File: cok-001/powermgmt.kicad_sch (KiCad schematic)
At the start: 87 parts, among them J6004 +12V_MAIN, J6005 +5V_EVER, Q6001 FDQ7238AS, Q6002 FDQ7238AS, Q6003 DTC144E, Q6004 SI3493, Q6006 UMH2NTN, Q6007 SI3493, Q6008 SI3493, Q6009 UMH2NTN, Q6010 SI4943, Q6012 Si3460DV, U6003 MB39A, U6004 PST3642UL, U6005 NCP511SN33T1G, U6006 NCP511SN18T1, U6007 TPS73101DBV, U6008 NCP511SN18T1, U6009 NCP511SN33T1G, U6011 NCP511, U6012 MM3141, U6013 MM1562, U6014 MM1591, U6017 BD3521, U6019 NCP511SN18T1, U6021 MM1591, U6022 MM1593, U6023 PST3642UL

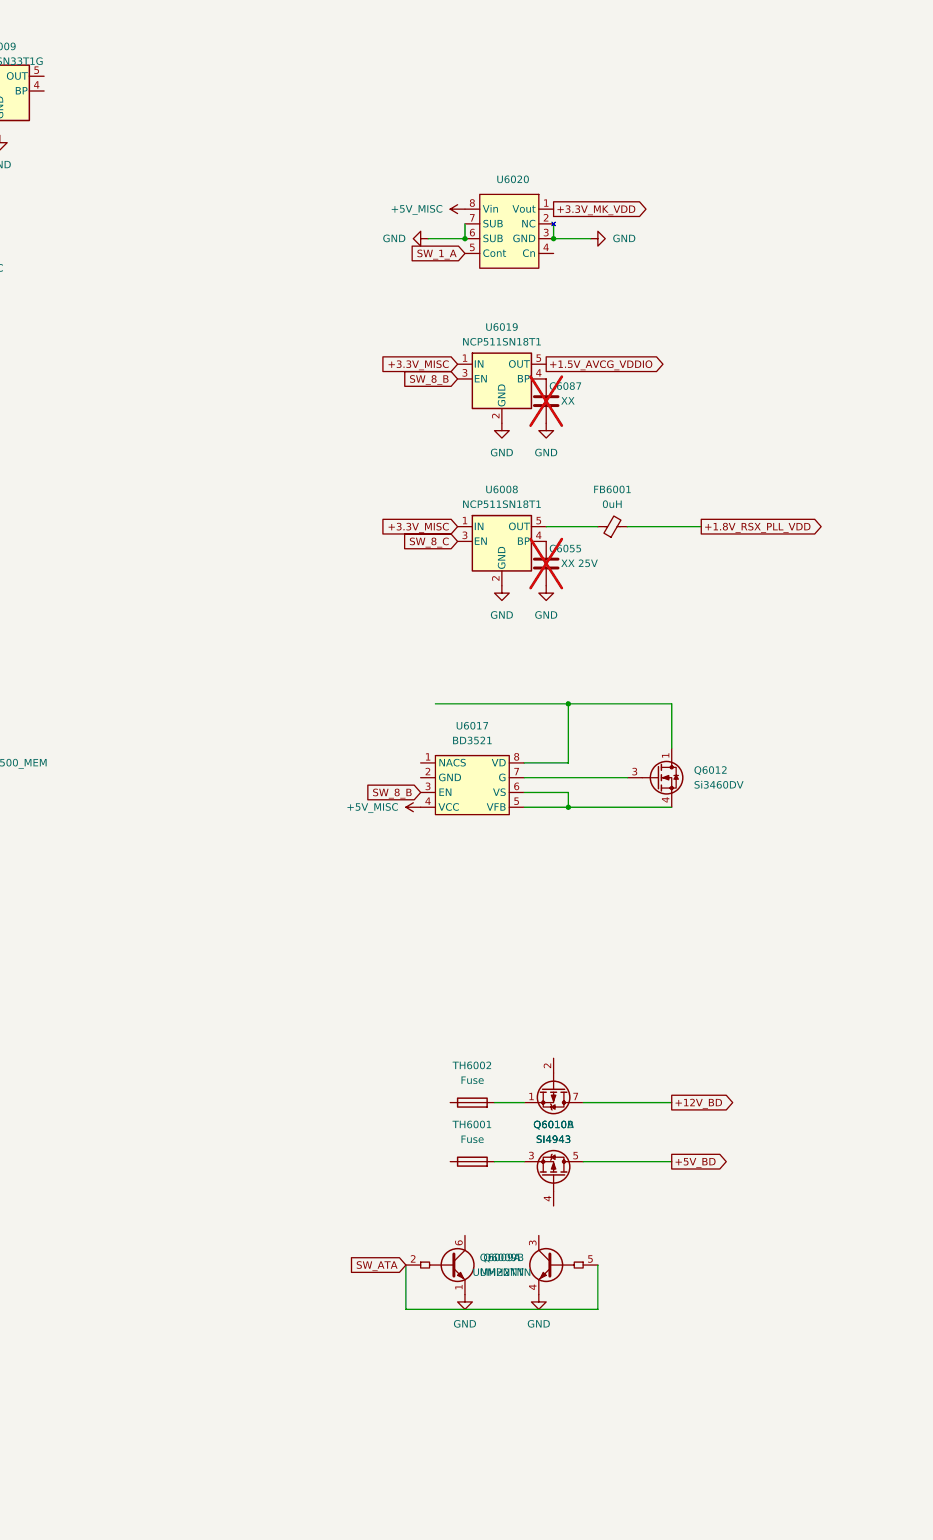
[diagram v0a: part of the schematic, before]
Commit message: caps
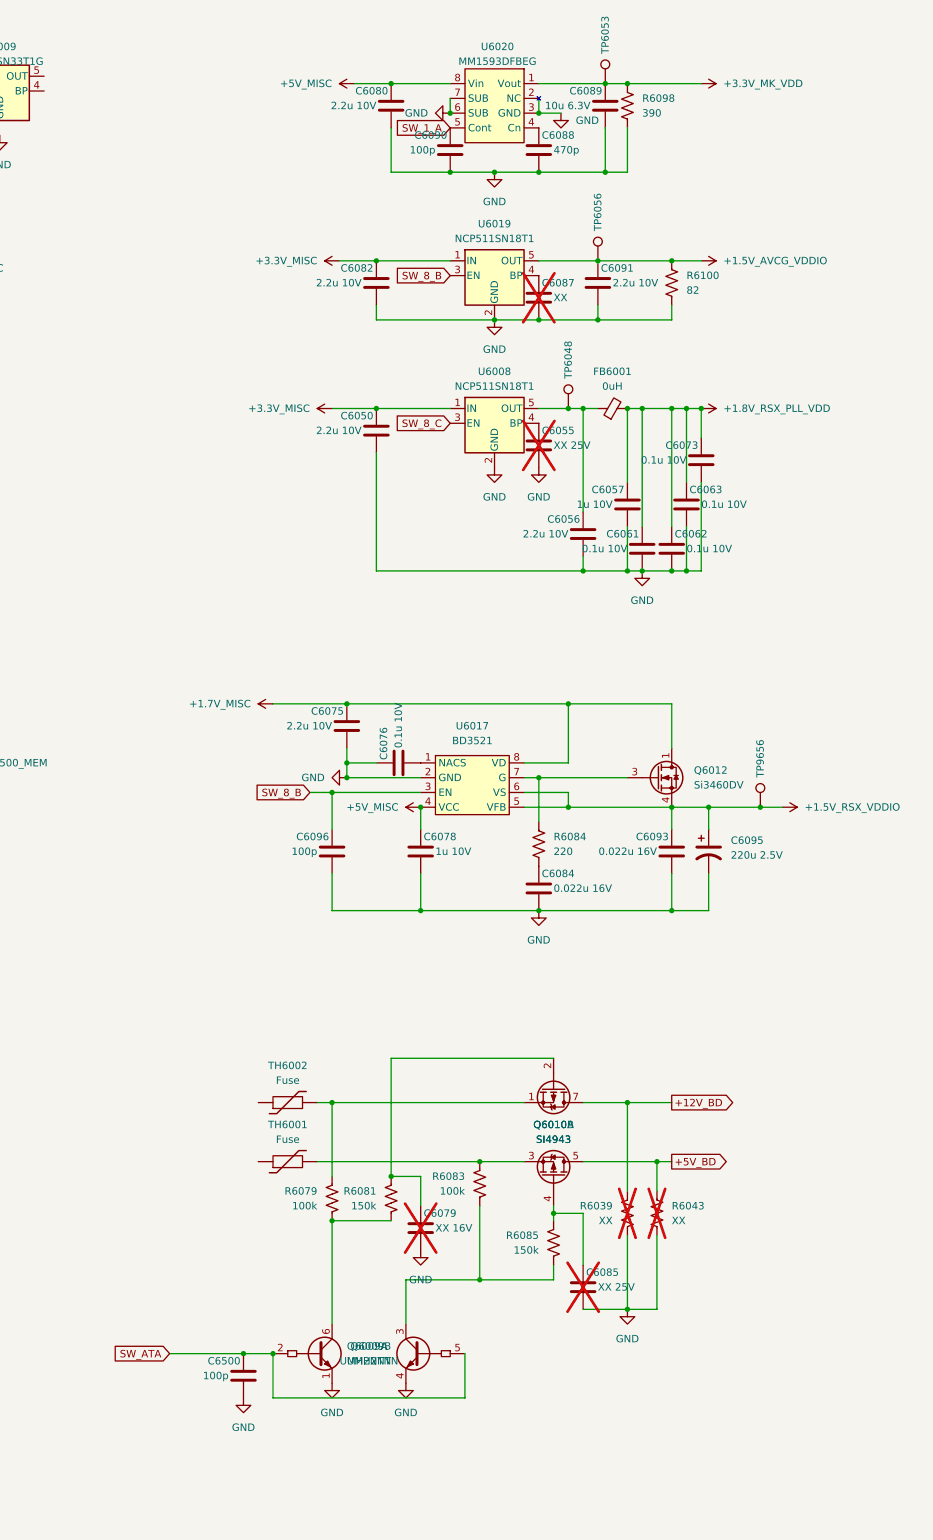
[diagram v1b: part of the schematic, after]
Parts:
- added C6050, C6056, C6075, C6080, C6082, C6091: 2.2u 10V, Capacitor_SMD:C_0805_2012Metric, symbol Device:C
- added C6057, C6078: 1u 10V, Capacitor_SMD:C_0402_1005Metric, symbol Device:C
- added C6061, C6062, C6063, C6073, C6076: 0.1u 10V, Capacitor_SMD:C_0402_1005Metric, symbol Device:C
- added C6079: XX 16V, Capacitor_SMD:C_0402_1005Metric, symbol Device:C
- added C6084, C6093: 0.022u 16V, Capacitor_SMD:C_0402_1005Metric, symbol Device:C
- added C6085: XX 25V, Capacitor_SMD:C_0402_1005Metric, symbol Device:C
- added C6088: 470p, Capacitor_SMD:C_0402_1005Metric, symbol Device:C
- added C6089: 10u 6.3V, Capacitor_SMD:C_0805_2012Metric, symbol Device:C
- added C6090, C6096, C6500: 100p, Capacitor_SMD:C_0402_1005Metric, symbol Device:C
- added C6095: 220u 2.5V, Capacitor_Tantalum_SMD:CP_EIA-3528-21_Kemet-B, symbol Device:C_Polarized_US
- added R6039, R6043: XX, Resistor_SMD:R_0402_1005Metric, symbol Device:R_US
- added R6079, R6083: 100k, Resistor_SMD:R_0402_1005Metric, symbol Device:R_US
- added R6081, R6085: 150k, Resistor_SMD:R_0402_1005Metric, symbol Device:R_US
- added R6084: 220, Resistor_SMD:R_0402_1005Metric, symbol Device:R_US
- added R6098: 390, Resistor_SMD:R_0402_1005Metric, symbol Device:R_US
- added R6100: 82, Resistor_SMD:R_0402_1005Metric, symbol Device:R_US
- added TP6048, TP6053, TP6056, TP9656: TestPoint, TestPoint:TestPoint_Pad_1.0x1.0mm, symbol Connector:TestPoint
- TH6001, TH6002: symbol Device:Fuse -> Device:Thermistor
- U6020: value ~ -> MM1593DFBEG
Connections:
- net +1.5V_AVCG_VDDIO: now also C6091.1, R6100.2, TP6056.1
- net +1.8V_RSX_PLL_VDD: now also C6057.1, C6061.1, C6062.1, C6063.1, C6073.1
- net +12V_BD: now also R6039.2
- net +3.3V_MISC: now also C6050.1, C6082.1
- net +3.3V_MK_VDD: now also C6089.1, R6098.2, TP6053.1
- net +5V_BD: now also R6043.2
- net +5V_MISC: now also C6078.1, C6080.1
- net GND: now also U6017.2 (GND), C6050.2, C6056.2, C6057.2, C6061.2, C6062.2, C6063.2, C6073.2, C6075.2, C6076.1, C6078.2, C6079.2, C6080.2, C6082.2, C6084.2, C6085.2, C6088.2, C6089.2, C6090.2, C6091.2, C6093.2, C6095.2, C6096.2, C6500.2, R6039.1, R6043.1, R6098.1, R6100.1
- net SW_1_A: now also C6090.1
- net SW_8_B: now also C6096.1
- net SW_ATA: now also C6500.1
- net +1.7V_MISC: now reaches Q6012.1 (D), Q6012.2 (D), Q6012.5 (D), Q6012.6 (D), U6017.8 (VD)
- net +1.7V_MISC: now also C6075.1
- net at Q6012.3 (G), U6017.7 (G): now also R6084.2
- net +1.5V_RSX_VDDIO: now reaches Q6012.4 (S), U6017.5 (VFB), U6017.6 (VS)
- net +1.5V_RSX_VDDIO: now also C6093.1, C6095.1, TP9656.1
- net at Q6010.3 (S2), TH6001.2: now also R6083.2
- net at Q6010.4 (G2): now also C6085.1, R6085.2
- net at Q6010.1 (S1), TH6002.2: now also R6079.2
- net at Q6010.2 (G1): now also C6079.1, R6081.2
- net at U6020.4 (Cn): now also C6088.1
- net at FB6001.1, U6008.5 (OUT): now also C6056.1, TP6048.1
- net at U6017.1 (NACS): now also C6076.2
- net at Q6009.6 (C1): now also R6079.1, R6081.1
- net at Q6009.3 (C2): now also R6083.1, R6085.1
- new net: C6084.1, R6084.1
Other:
- moved on the sheet: C6055, C6087, FB6001, Q6009A, Q6009B, TH6001, TH6002, U6008, U6019, U6020
